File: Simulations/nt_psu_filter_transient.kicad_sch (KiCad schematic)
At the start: 22 parts

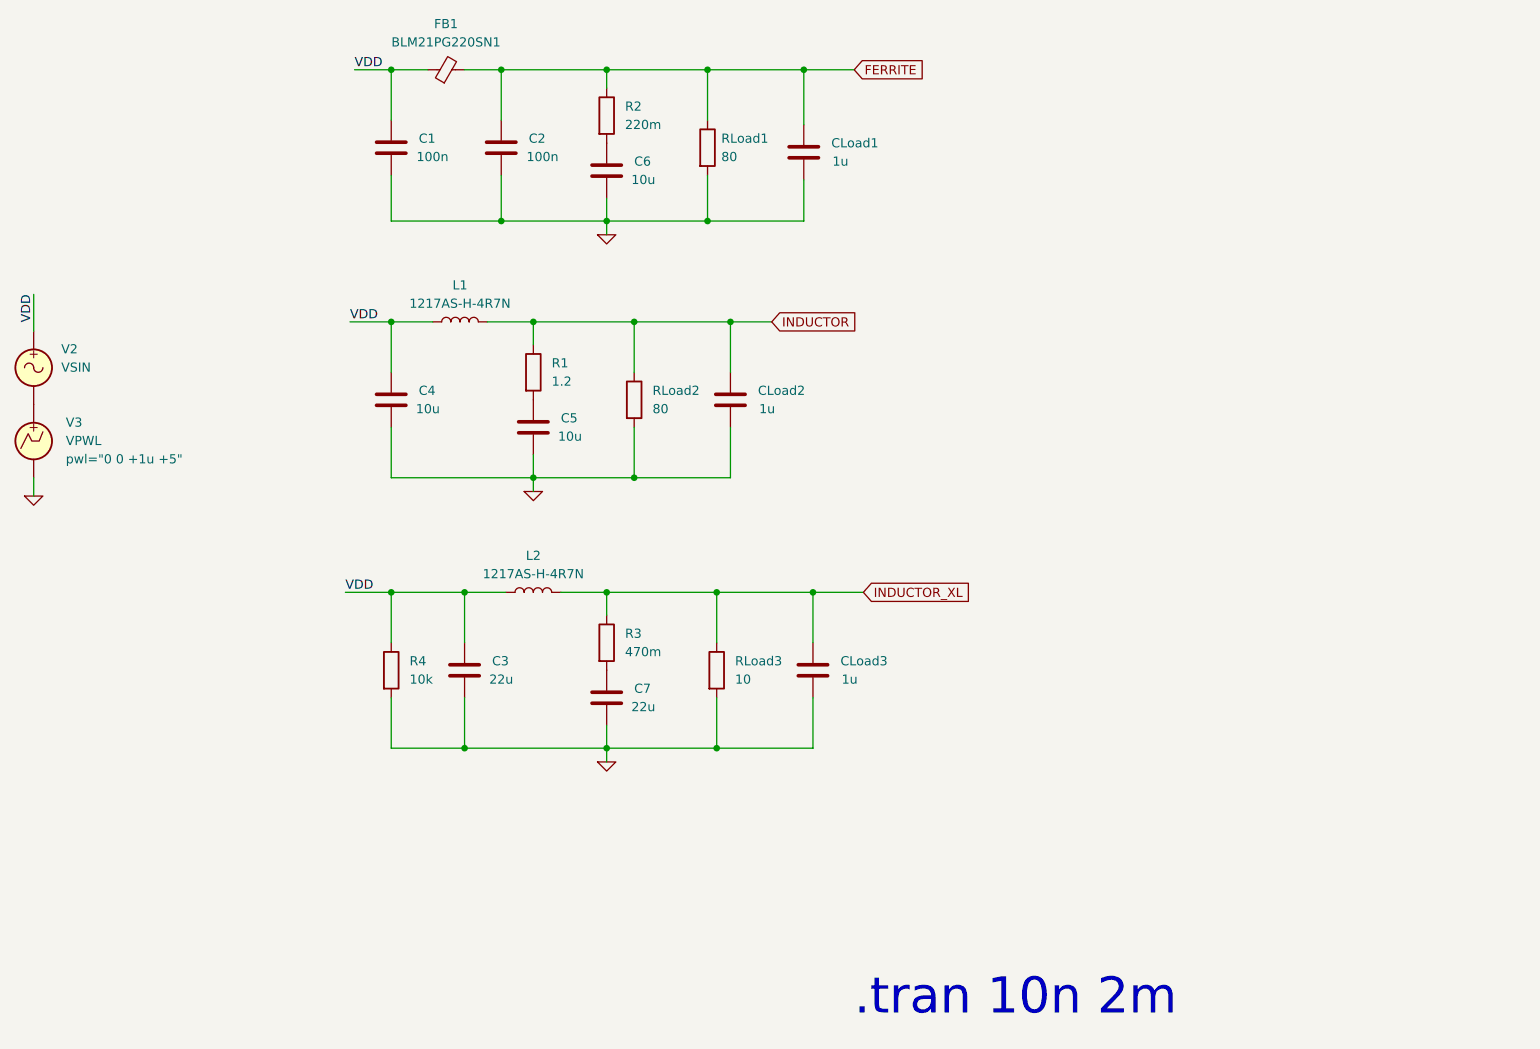
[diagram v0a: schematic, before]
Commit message: power supply simulations
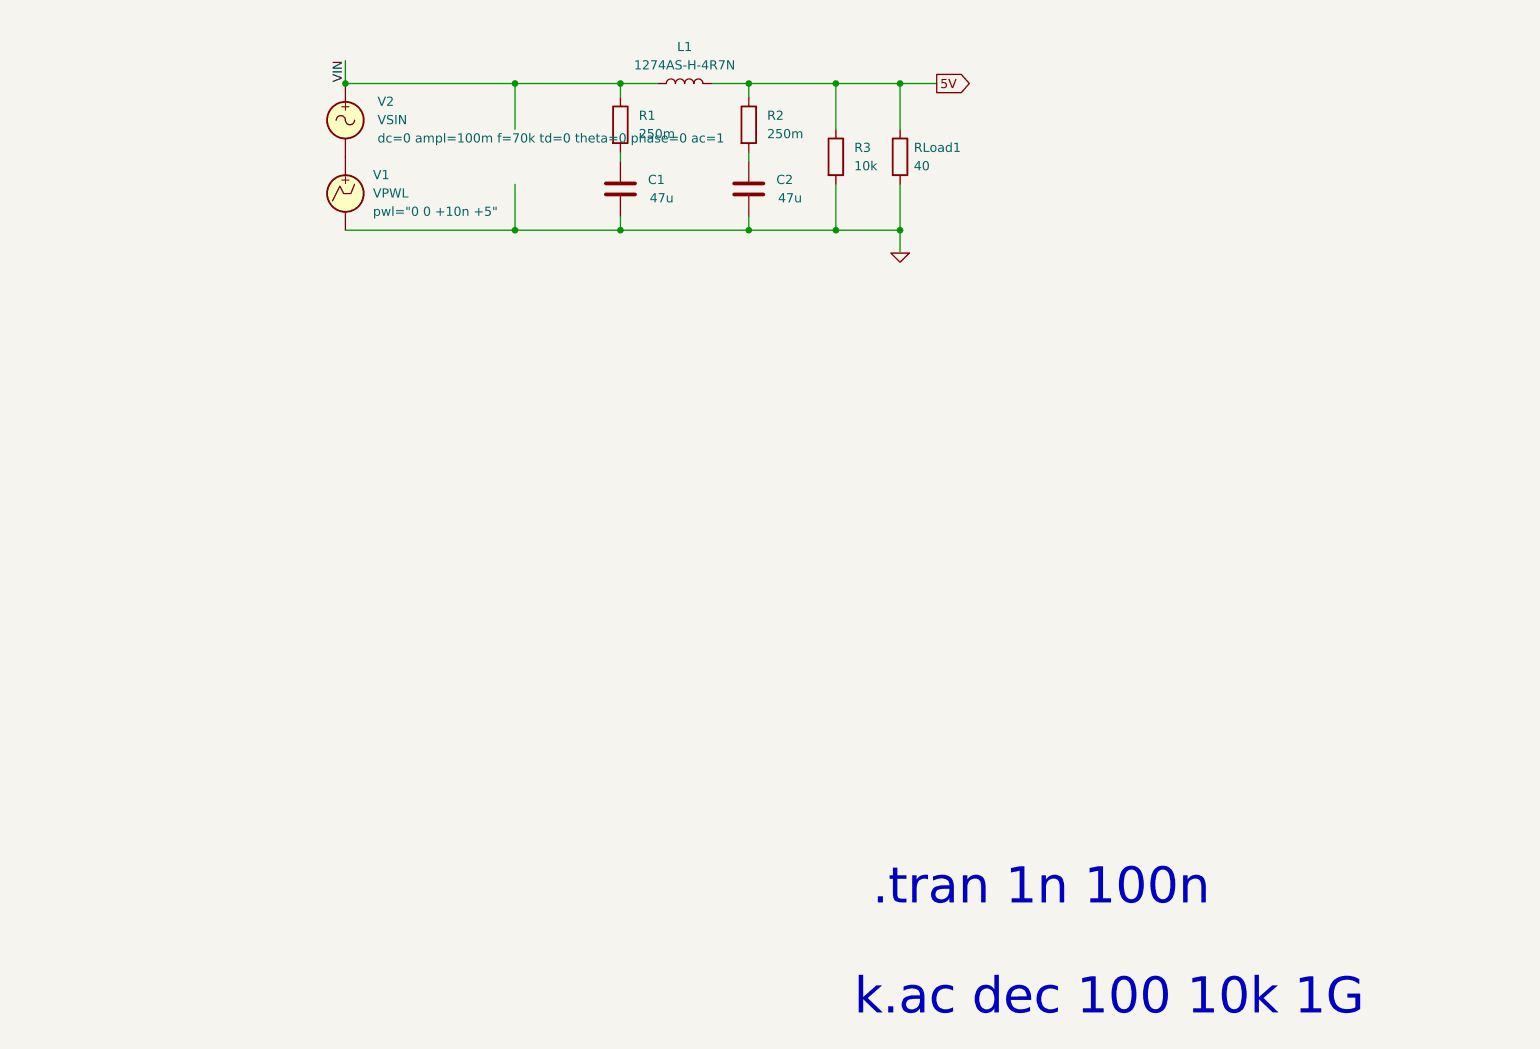
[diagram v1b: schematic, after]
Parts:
- removed C3, C4, C5, C6, C7, CLoad1, CLoad2, CLoad3: ${SIM.PARAMS}, symbol Device:C
- removed FB1: BLM21PG220SN1, symbol Device:FerriteBead_Small
- removed L2: ${SIM.PARAMS}, symbol Device:L
- removed R4: 10k, symbol Device:R
- removed RLoad2: 80, symbol Device:R
- removed RLoad3: 10, symbol Device:R
- removed V3: VPWL, symbol Simulation_SPICE:VPWL
- added V1: VPWL, symbol Simulation_SPICE:VPWL
- R1: value 1.2 -> 250m
- R2: value 220m -> 250m
- R3: value 470m -> 10k
- RLoad1: value 80 -> 40
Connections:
- net INDUCTOR_XL is gone; now on net 5V: R3.1
- net 0: now also R3.2, V1.2
- net at R2.2: now also C2.1
- net at R1.2: now also C1.1
- net at V2.2: now also V1.1
- net FERRITE renamed 5V
- net 5V: now also L1.2; no longer C2.1
- net INDUCTOR renamed VIN
- net VIN: now also L1.1, V2.1; no longer L1.2
- removed net VDD: C1.1, L1.1, V2.1
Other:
- note added: ".tran 1n 100n"
- note added: "k.ac dec 100 10k 1G"
- note removed: ".tran 10n 2m"
